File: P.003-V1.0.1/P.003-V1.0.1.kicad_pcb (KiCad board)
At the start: 2 copper layers, 42 x 78.5 mm, 21 parts, among them Q1 BS250, SW1 ON/OFF, SW2 Mode, SW3 Roll, U1 ATtiny85-20P, U2 74HC595

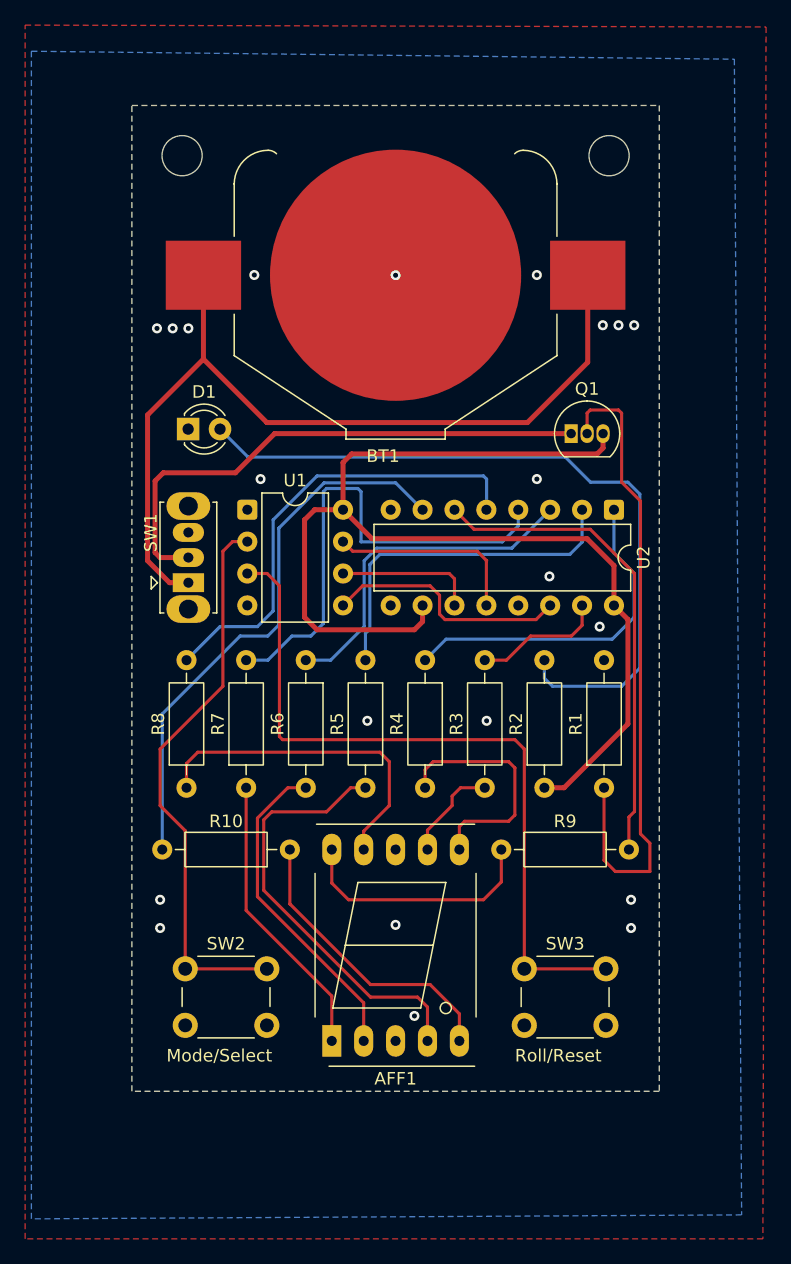
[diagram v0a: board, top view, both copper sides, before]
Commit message: add files
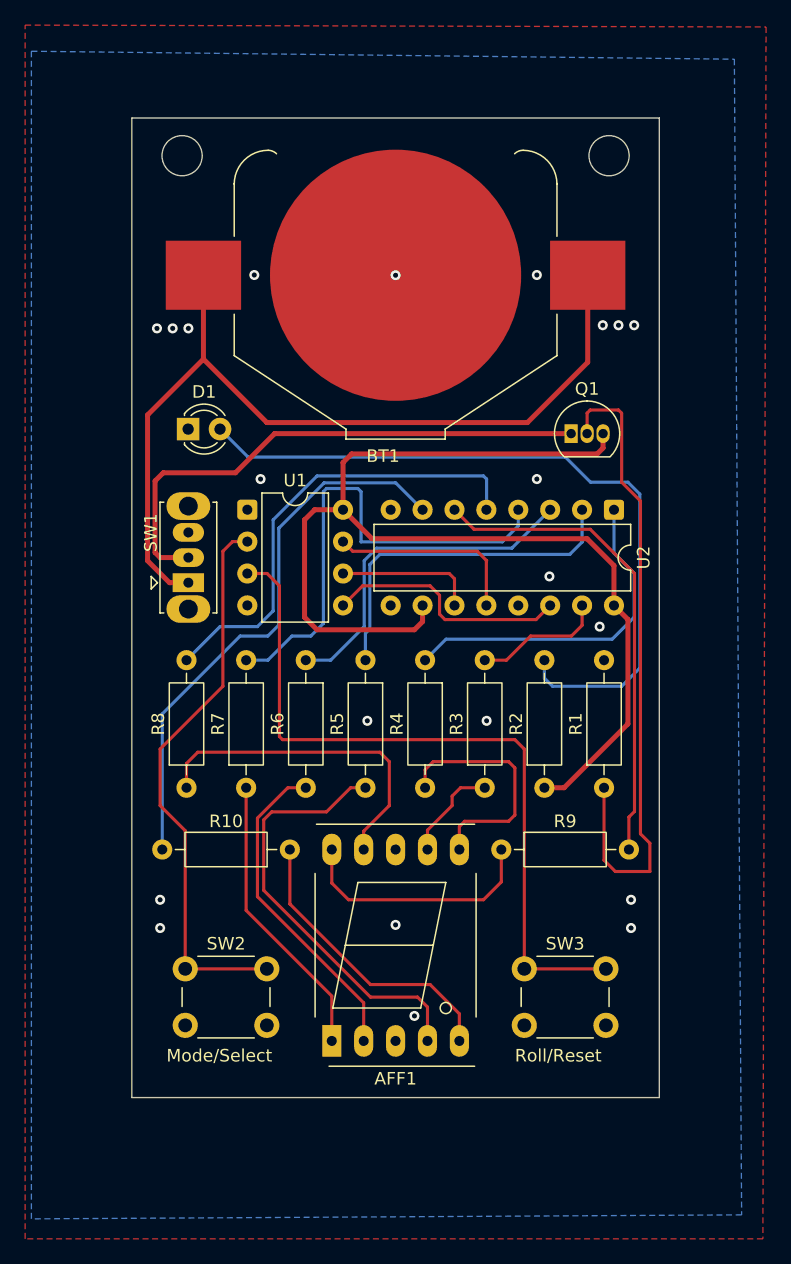
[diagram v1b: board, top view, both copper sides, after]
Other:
- board size 42 x 78.5 mm -> 42 x 78 mm
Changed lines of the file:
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@@
 	)
 	(gr_rect
-		(start 108 47.98)
-		(end 150 126.48)
+		(start 108 48.98)
+		(end 150 126.98)
 		(radius 4)
 		(stroke
 			(width 0.05)
-			(type dash_dot)
+			(type solid)
 		)
 		(fill no)

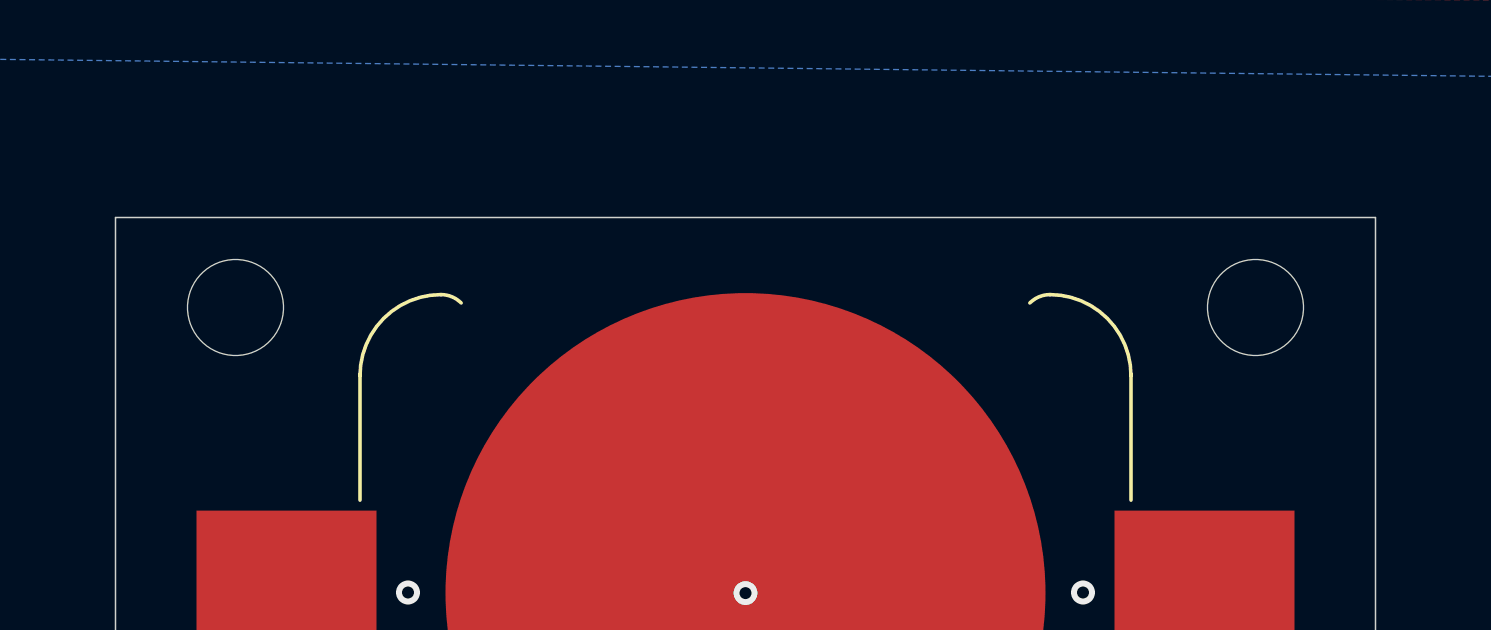
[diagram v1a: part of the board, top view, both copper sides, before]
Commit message: ok
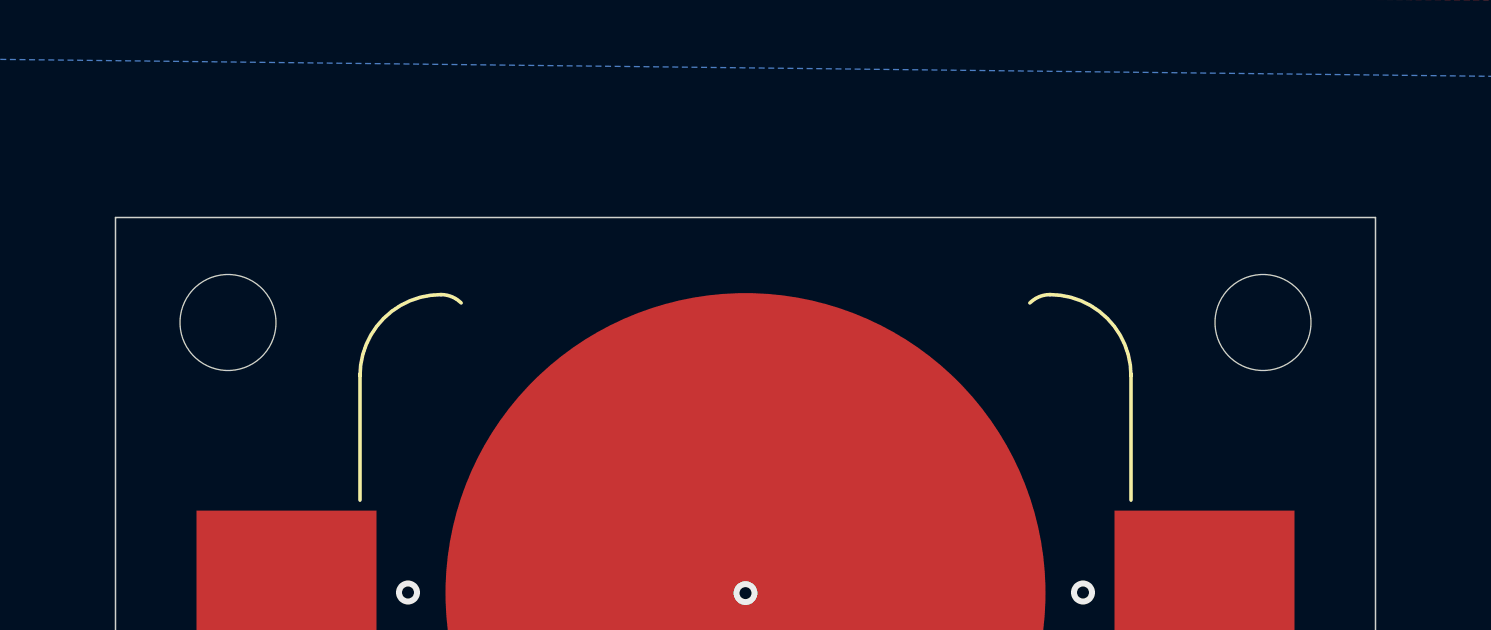
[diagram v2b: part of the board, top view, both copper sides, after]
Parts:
- moved ? 0.56 mm to (111.8, 52.5)
- moved ? 0.56 mm to (146.2, 52.5)
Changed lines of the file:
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@@
 			(drillshape 0)
 			(scaleselection 1)
-			(outputdirectory "../File_Manufacturing/")
+			(outputdirectory "../Manufacturing/")
 		)
 	)
@@
 		(locked yes)
 		(layer "F.Cu")
-		(at 112 51.98)
+		(at 111.75 52.48)
 		(descr "Mounting Hole 3.2mm, M3, no annular, generated by kicad-footprint-generator mountinghole.py")
 		(tags "mountinghole M3")
@@
 		(locked yes)
 		(layer "F.Cu")
-		(at 146 51.98)
+		(at 146.25 52.48)
 		(descr "Mounting Hole 3.2mm, M3, no annular, generated by kicad-footprint-generator mountinghole.py")
 		(tags "mountinghole M3")
